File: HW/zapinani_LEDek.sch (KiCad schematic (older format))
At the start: 4 parts, among them Q3 Q_PMOS_DGS, Q4 Q_PMOS_DGS

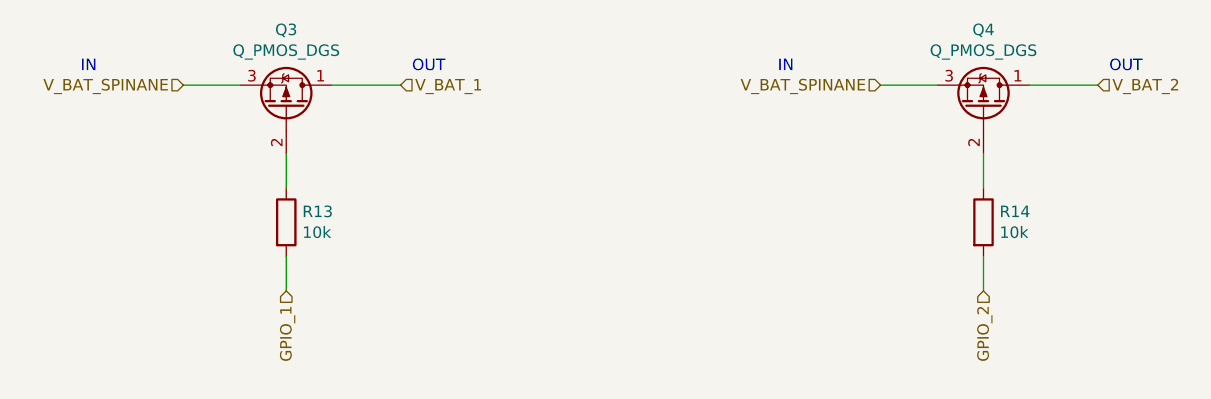
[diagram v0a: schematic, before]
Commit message: repair project
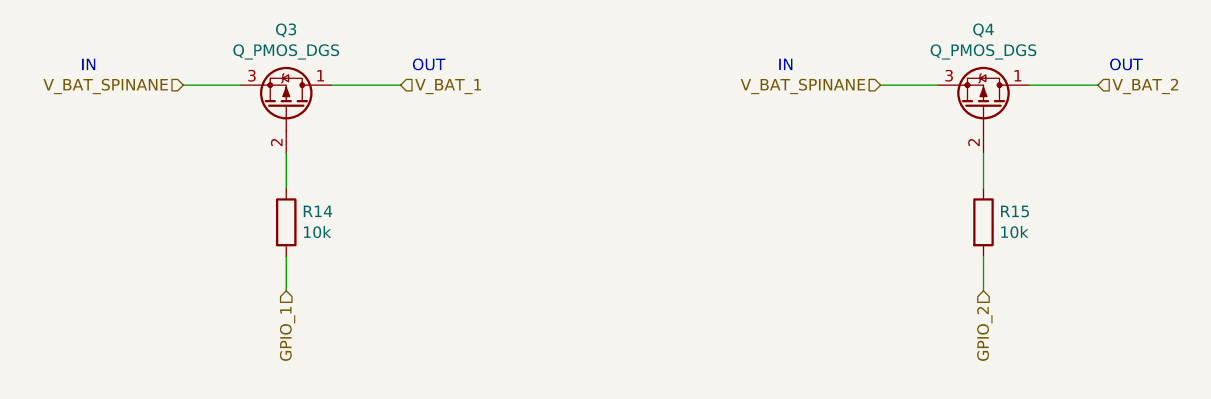
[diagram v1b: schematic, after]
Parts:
- renumbered R13 to R14, R14 to R15
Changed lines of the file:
@@
 P 2650 3800
 AR Path="/5F8EC656" Ref="R?"  Part="1"
-AR Path="/5F7BA54B/5F8EC656" Ref="R13"  Part="1"
+AR Path="/5F7BA54B/5F8EC656" Ref="R14"  Part="1"
 AR Path="/5F7BA54B/5F7BCB45/5F8EC656" Ref="R?"  Part="1"
 AR Path="/5F7BA54B/5F7BCBA6/5F8EC656" Ref="R?"  Part="1"
 AR Path="/5F7BA54B/5F7BCC0A/5F8EC656" Ref="R?"  Part="1"
 AR Path="/5F7BA54B/5F7BCC69/5F8EC656" Ref="R?"  Part="1"
-F 0 "R13" H 2720 3846 50  0000 L CNN
+F 0 "R14" H 2720 3846 50  0000 L CNN
 F 1 "10k" H 2720 3755 50  0000 L CNN
 F 2 "Resistor_SMD:R_0402_1005Metric" V 2580 3800 50  0001 C CNN
@@
 	0    1    -1   0
 $EndComp
-$Comp
-L Device:R R?
-U 1 1 5F8ECA6B
-P 5700 3800
-AR Path="/5F8ECA6B" Ref="R?"  Part="1"
-AR Path="/5F7BA54B/5F8ECA6B" Ref="R14"  Part="1"
-AR Path="/5F7BA54B/5F7BCB45/5F8ECA6B" Ref="R?"  Part="1"
-AR Path="/5F7BA54B/5F7BCBA6/5F8ECA6B" Ref="R?"  Part="1"
-AR Path="/5F7BA54B/5F7BCC0A/5F8ECA6B" Ref="R?"  Part="1"
-AR Path="/5F7BA54B/5F7BCC69/5F8ECA6B" Ref="R?"  Part="1"
-F 0 "R14" H 5770 3846 50  0000 L CNN
-F 1 "10k" H 5770 3755 50  0000 L CNN
-F 2 "Resistor_SMD:R_0402_1005Metric" V 5630 3800 50  0001 C CNN
-F 3 "~" H 5700 3800 50  0001 C CNN
-F 4 "C25744" H 5700 3800 50  0001 C CNN "LCSC"
-	1    5700 3800
-	1    0    0    -1
-$EndComp
 Wire Wire Line
 	5250 3200 5500 3200
@@
 Text Notes 6250 3150 0    50   ~ 0
 OUT\n
+$Comp
+L Device:R R?
+U 1 1 5F8ECA6B
+P 5700 3800
+AR Path="/5F8ECA6B" Ref="R?"  Part="1"
+AR Path="/5F7BA54B/5F8ECA6B" Ref="R15"  Part="1"
+AR Path="/5F7BA54B/5F7BCB45/5F8ECA6B" Ref="R?"  Part="1"
+AR Path="/5F7BA54B/5F7BCBA6/5F8ECA6B" Ref="R?"  Part="1"
+AR Path="/5F7BA54B/5F7BCC0A/5F8ECA6B" Ref="R?"  Part="1"
+AR Path="/5F7BA54B/5F7BCC69/5F8ECA6B" Ref="R?"  Part="1"
+F 0 "R15" H 5770 3846 50  0000 L CNN
+F 1 "10k" H 5770 3755 50  0000 L CNN
+F 2 "Resistor_SMD:R_0402_1005Metric" V 5630 3800 50  0001 C CNN
+F 3 "~" H 5700 3800 50  0001 C CNN
+F 4 "C25744" H 5700 3800 50  0001 C CNN "LCSC"
+	1    5700 3800
+	1    0    0    -1
+$EndComp
 $EndSCHEMATC
